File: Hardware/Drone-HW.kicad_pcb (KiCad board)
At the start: 2 copper layers, 62.5 x 42 mm, 30 parts, among them Con5 espTool_conn, J1 Conn_01x03, J2 Conn_01x03, J3 Conn_01x03, J4 Conn_01x03, J5 Conn_01x02_Pin, Q5 BC846, Q6 BC846, SW3 Tactile, U1 ESP32-WROOM-32D, U2 U2, U3 NRF24L01_Breakout

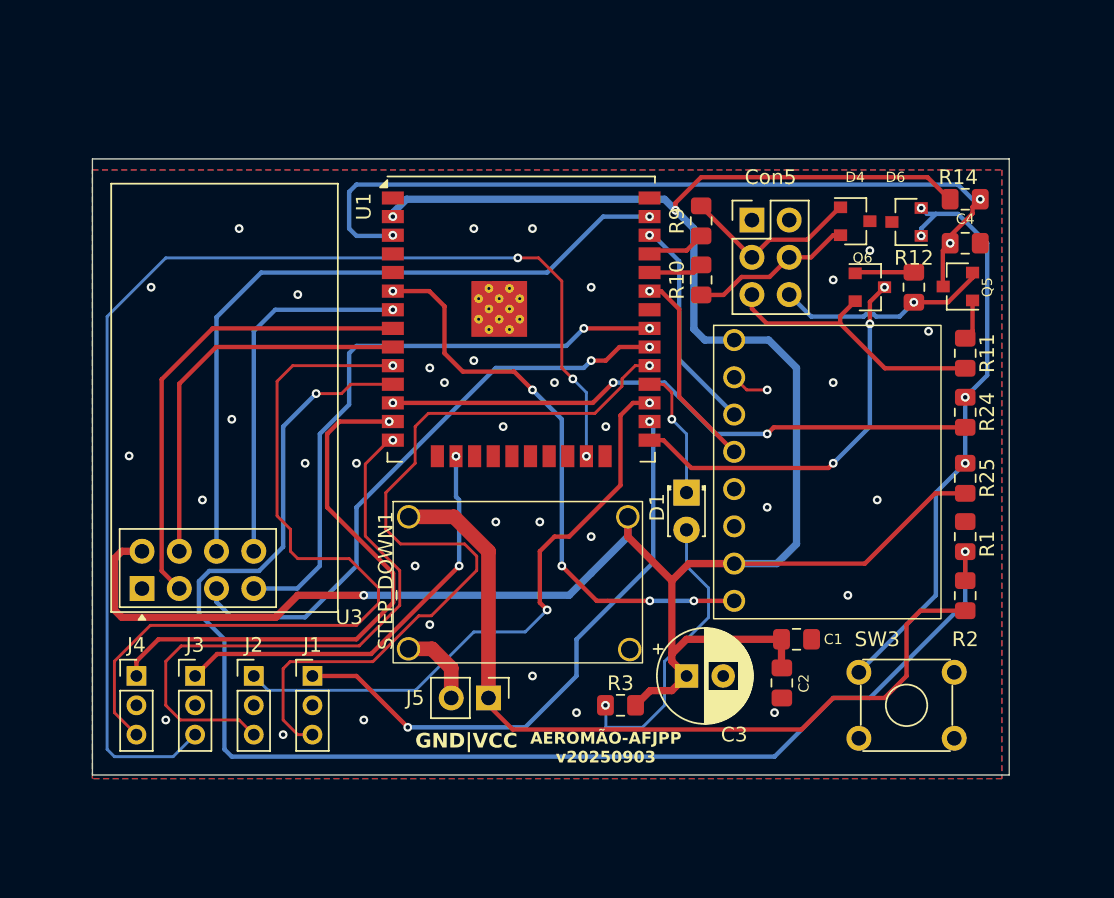
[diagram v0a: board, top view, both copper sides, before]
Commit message: Dando push na versão final de hardware
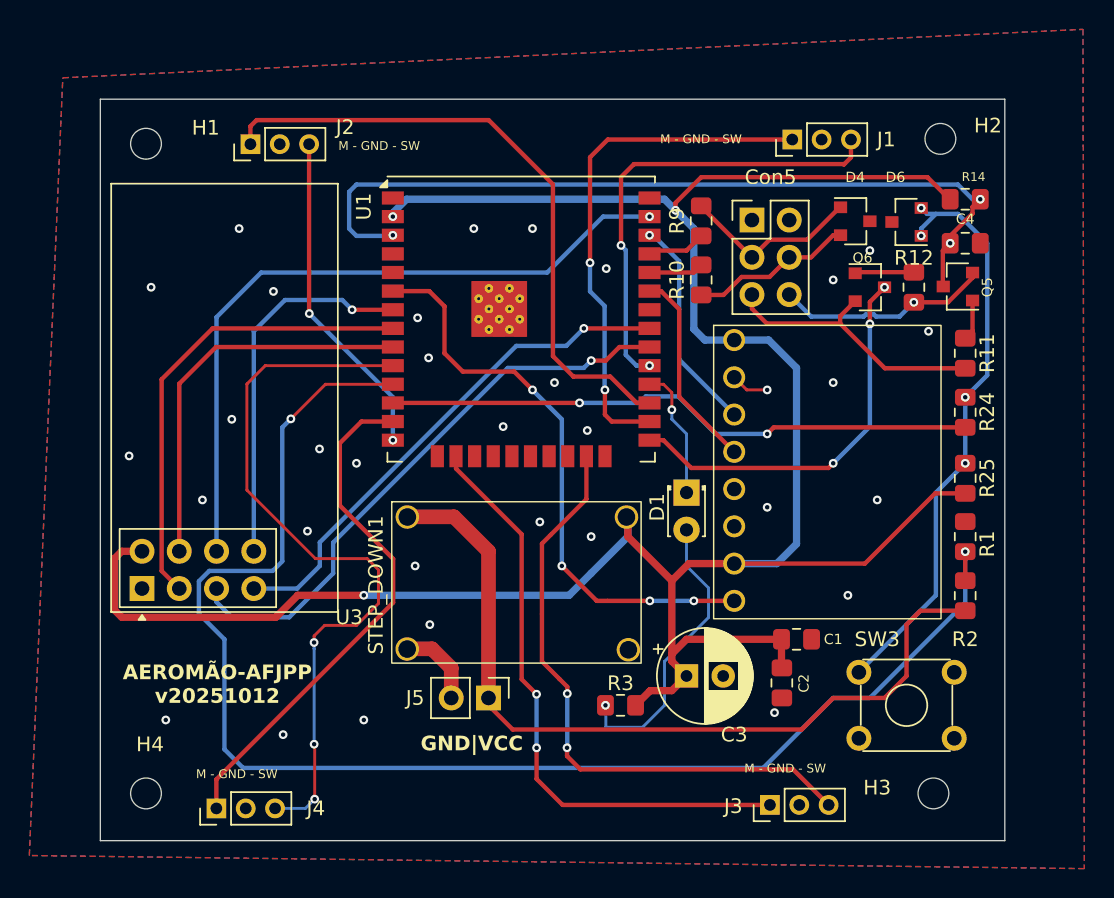
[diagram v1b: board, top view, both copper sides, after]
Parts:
- added H1: MountingHole, MountingHole:MountingHole_2.1mm, F.Cu at (137.2, 32.2)
- added H2: MountingHole, MountingHole:MountingHole_2.1mm, F.Cu at (191.3, 31.9)
- added H3: MountingHole, MountingHole:MountingHole_2.1mm, F.Cu at (190.8, 76.5)
- added H4: MountingHole, MountingHole:MountingHole_2.1mm, F.Cu at (137.2, 76.5)
- moved J1 49.1 mm to (181.2, 31.9), turned to 90 degrees
- moved J3 40.2 mm to (179.7, 77.3), turned to 90 degrees
- moved J2 36.3 mm to (144.3, 32.2), turned to 90 degrees
- moved J4 10.5 mm to (141.9, 77.5), turned to 90 degrees
- moved STEP_DOWN1 0.09 mm to (153.9, 56.6)
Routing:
- net /sw3: track 82.3 -> 41.6 mm, vias 3 -> 2
- net /sw1: track 55.6 -> 31.7 mm, vias 1 -> 2
- net /sw2: track 40.5 -> 22.8 mm, vias 1 -> 2
- net /Motor3: track 28.7 -> 40.9 mm
- net /MISO: track 41.6 -> 35.3 mm, vias 2 -> 1
- net /Motor1: track 40.5 -> 35.5 mm
- net /sw4: track 53.6 -> 50.6 mm, vias 1 -> 3
- net /Motor4: track 38.1 -> 35.4 mm, vias 1 -> 0
- net /Motor2: track 41.3 -> 43.4 mm, vias 2 -> 0
- net /V_Bat: track 96.3 -> 97.5 mm
- net /SCK: track 40.8 -> 39.7 mm, vias 2 -> 1
- net /B_START: track 41.2 -> 40.5 mm, vias 3 -> 2
- net /IRQ: track 25.1 -> 25.6 mm
- net GND: vias 36 -> 33
- net /SDA-SPU: vias 1 -> 0
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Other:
- board size 62.5 x 42 mm -> 61.7 x 50.5 mm
- board text added: "AEROMÃO-AFJPP v20251012"
- board text added: "M - GND - SW"
- board text removed: "AEROMÃO-AFJPP v20250903"
